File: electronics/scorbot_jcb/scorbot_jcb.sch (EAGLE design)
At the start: 13 parts

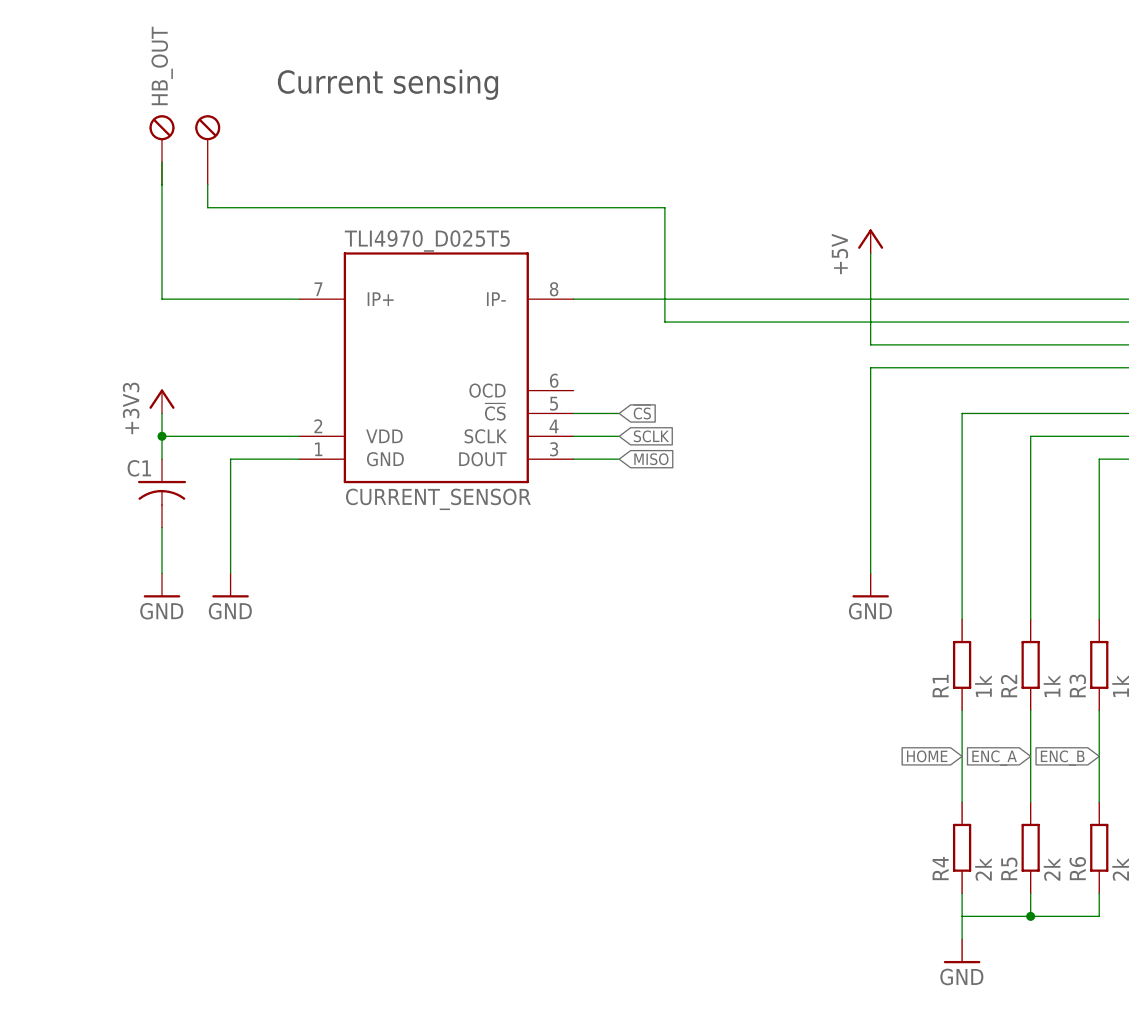
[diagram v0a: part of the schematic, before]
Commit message: Ruteo
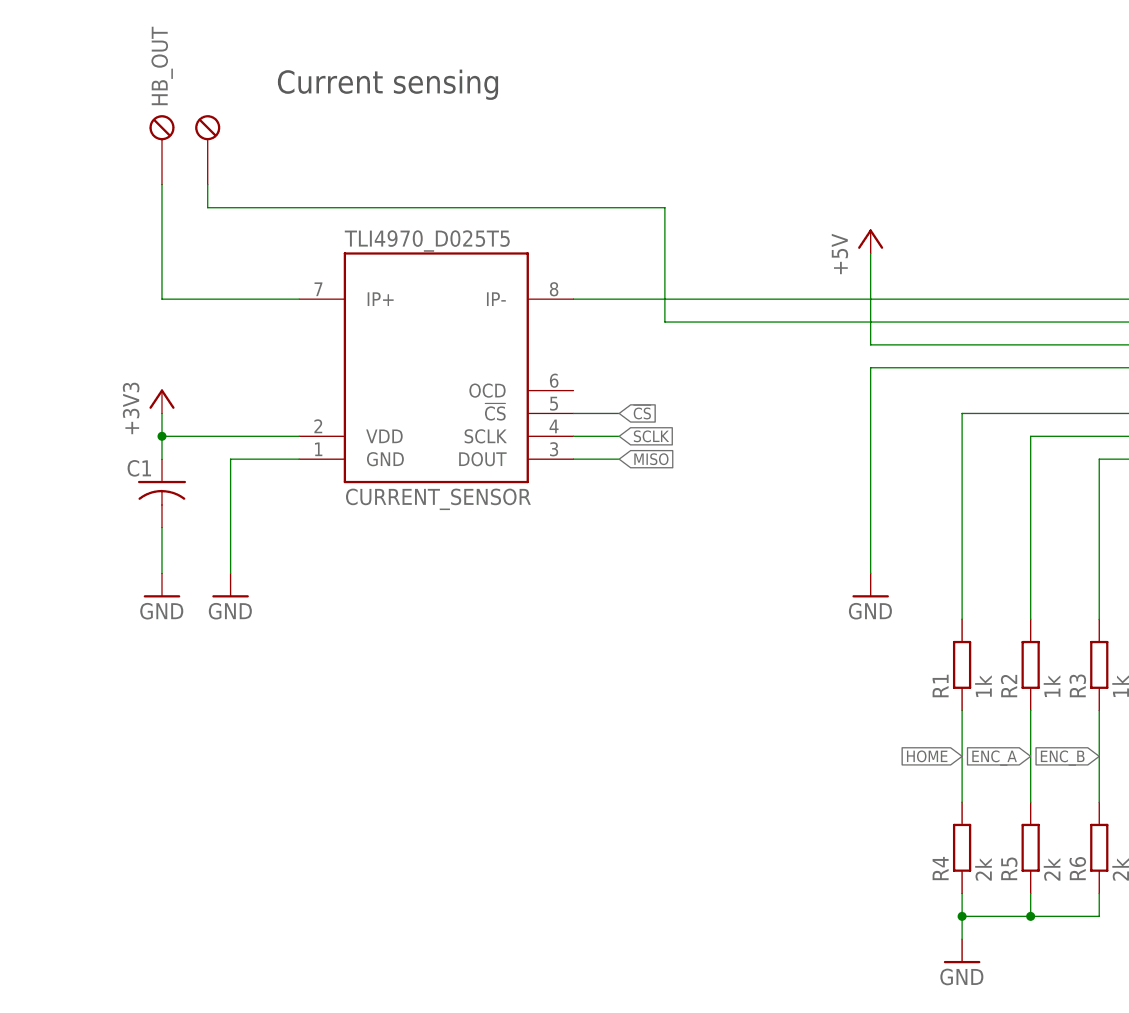
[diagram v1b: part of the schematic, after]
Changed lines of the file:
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@@
 <?xml version="1.0" encoding="utf-8"?>
 <!DOCTYPE eagle SYSTEM "eagle.dtd">
-<eagle version="7.6.0">
+<eagle version="7.4.0">
 <drawing>
 <settings>
@@
 <setting verticaltext="up"/>
 </settings>
-<grid distance="0.1" unitdist="inch" unit="inch" style="lines" multiple="1" display="yes" altdistance="0.01" altunitdist="inch" altunit="inch"/>
+<grid distance="0.1" unitdist="inch" unit="inch" style="lines" multiple="1" display="no" altdistance="0.01" altunitdist="inch" altunit="inch"/>
 <layers>
 <layer number="1" name="Top" color="4" fill="1" visible="no" active="no"/>
@@
 <pinref part="CURRENT_SENSOR" gate="G$1" pin="IP+"/>
 <wire x1="43.18" y1="121.92" x2="27.94" y2="121.92" width="0.1524" layer="91"/>
+<pinref part="HB_OUT" gate="G$1" pin="P1"/>
 <wire x1="27.94" y1="121.92" x2="27.94" y2="134.62" width="0.1524" layer="91"/>
-<pinref part="HB_OUT" gate="G$1" pin="P1"/>
-<wire x1="27.94" y1="134.62" x2="27.94" y2="137.16" width="0.1524" layer="91"/>
 </segment>
 </net>
@@
 <wire x1="132.08" y1="53.34" x2="124.46" y2="53.34" width="0.1524" layer="91"/>
 <junction x="124.46" y="53.34"/>
-</segment>
-<segment>
+<junction x="116.84" y="53.34"/>
+</segment>
+<segment>
